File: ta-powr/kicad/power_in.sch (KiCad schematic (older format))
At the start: 29 parts, among them U1 SPV1040, U3 TLV8544DT, U4 ADS1115-Q1

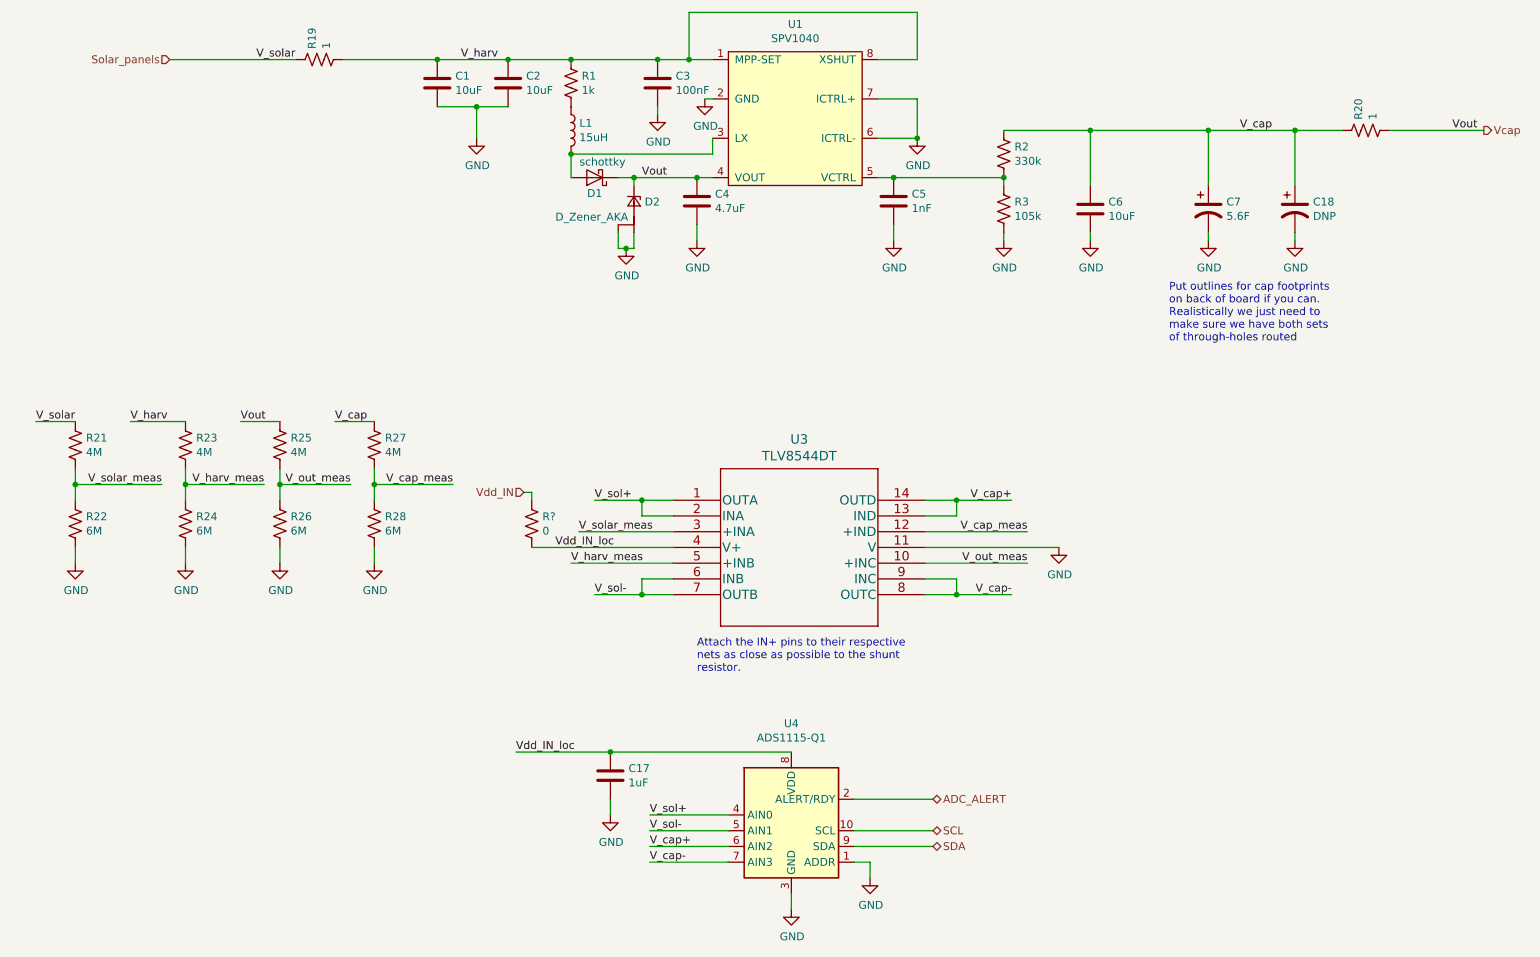
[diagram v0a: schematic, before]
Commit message: first crack at parts placement on power board
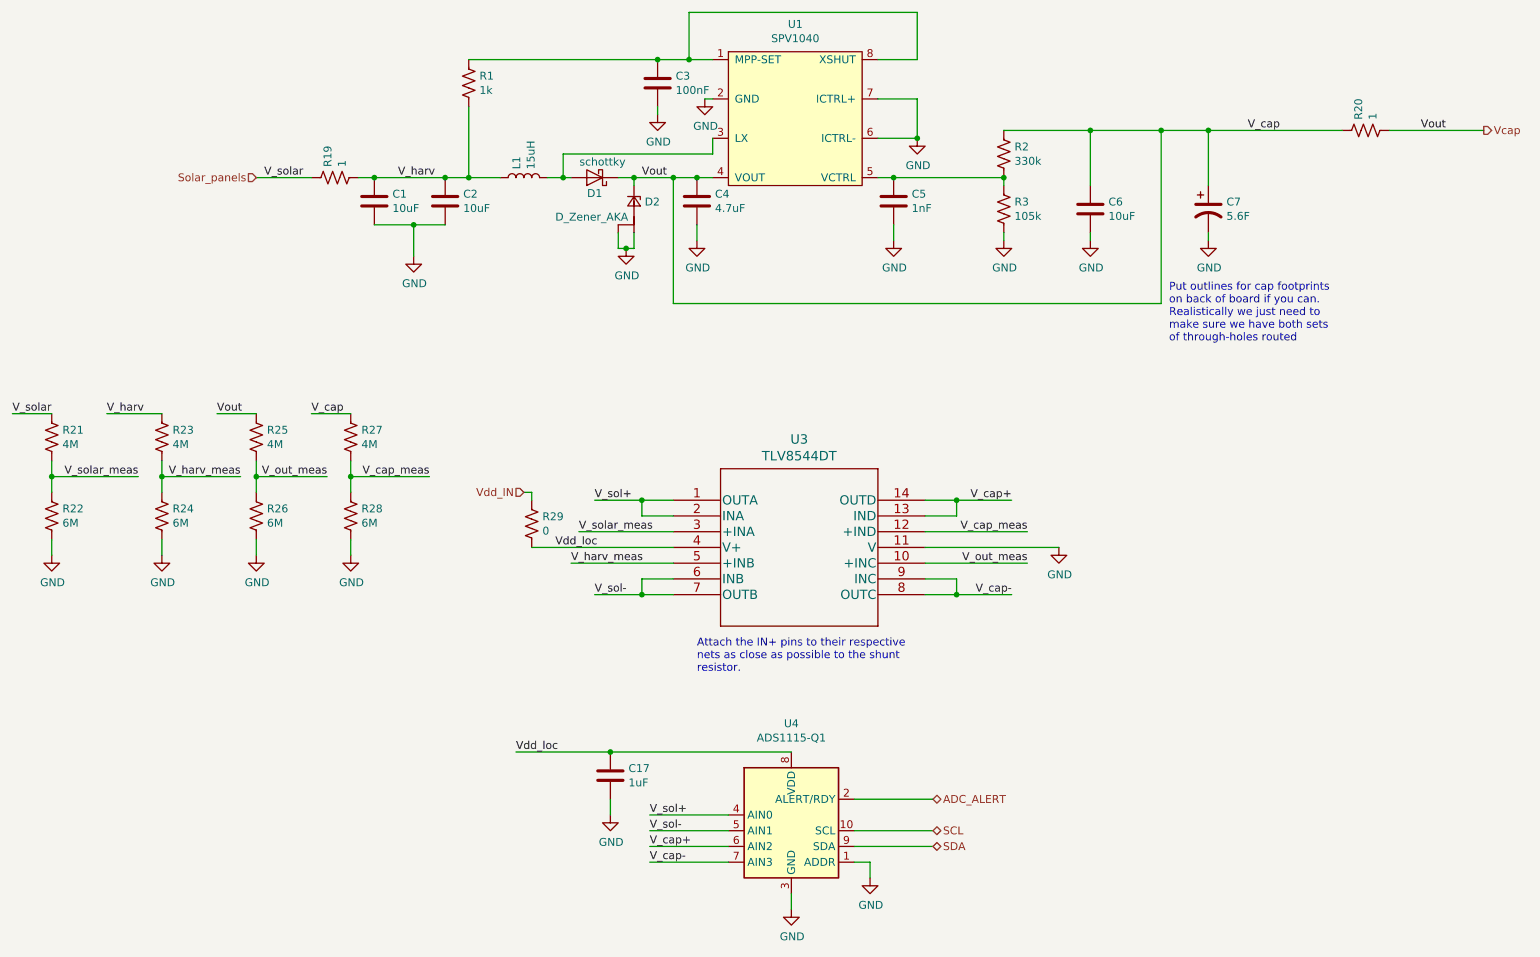
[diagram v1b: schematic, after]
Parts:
- removed C18: DNP, ta-powr:TECATE_PBL, symbol Device:CP1
- gave numbers to parts that had none: 1
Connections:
- net V_cap is gone; now on net Vcap: C6.1, C7.1, R2.1, R20.1, R27.1
- net V_harv: now also L1.1, R1.2; no longer C3.1, R1.1, U1.1 (MPP-SET), U1.8 (XSHUT)
- net Vdd_IN_loc renamed Vdd_loc
- new net: C3.1, R1.1, U1.1 (MPP-SET), U1.8 (XSHUT)
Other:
- moved on the sheet: C1, C2, L1, R1, R19, R21, R22, R23, R24, R25, R26, R27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
